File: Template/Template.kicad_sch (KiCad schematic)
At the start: 16 parts, among them J1 Conn_01x04, J2 Conn_01x04, J3 Conn_02x05_Odd_Even, J4 Conn_01x01, J6 Conn_02x05_Odd_Even, U1 PCA9535DBR

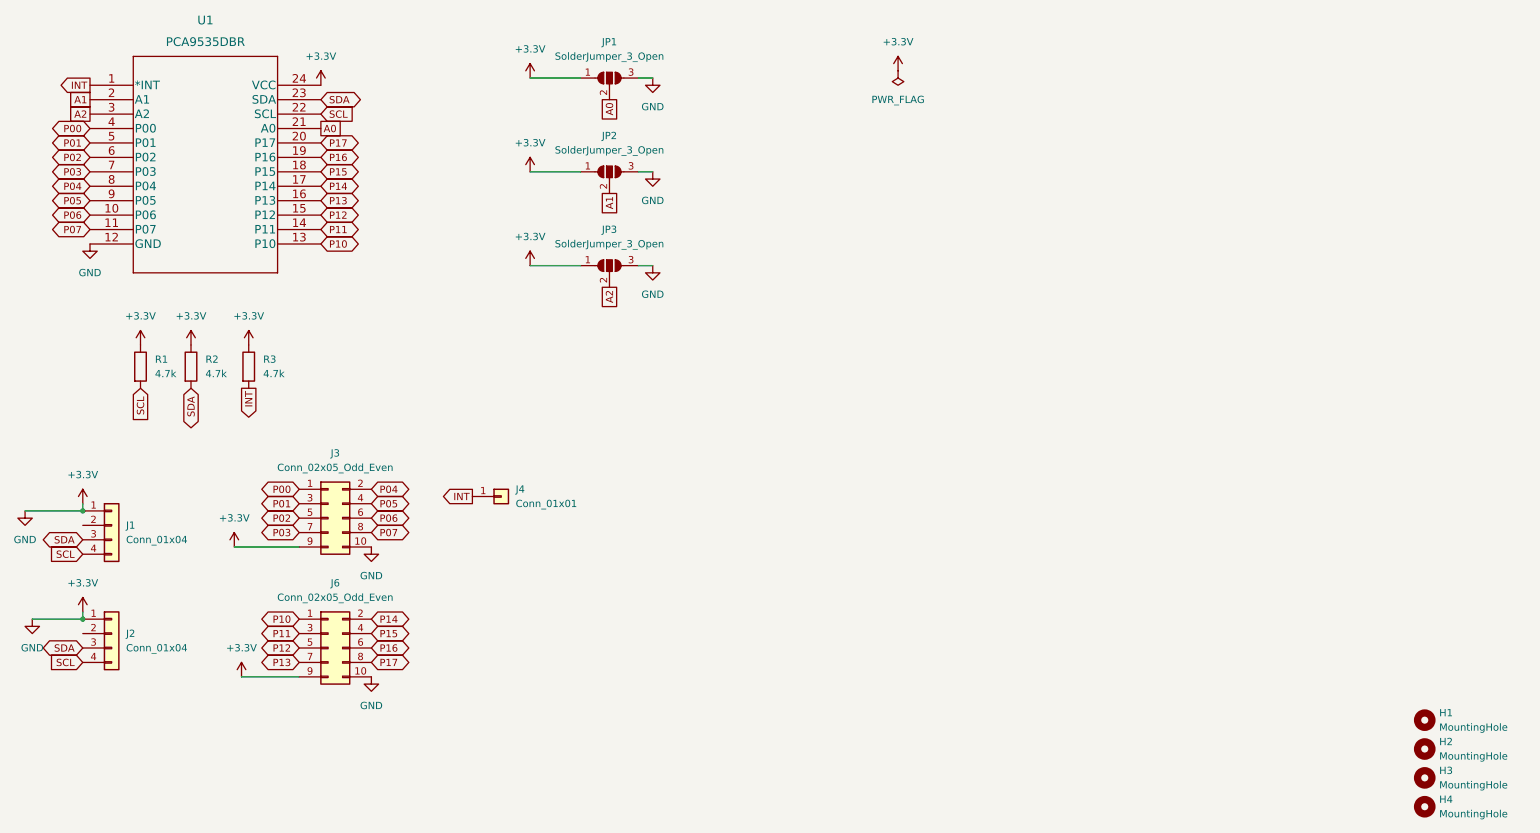
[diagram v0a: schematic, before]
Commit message: Futher Progress on the gpio
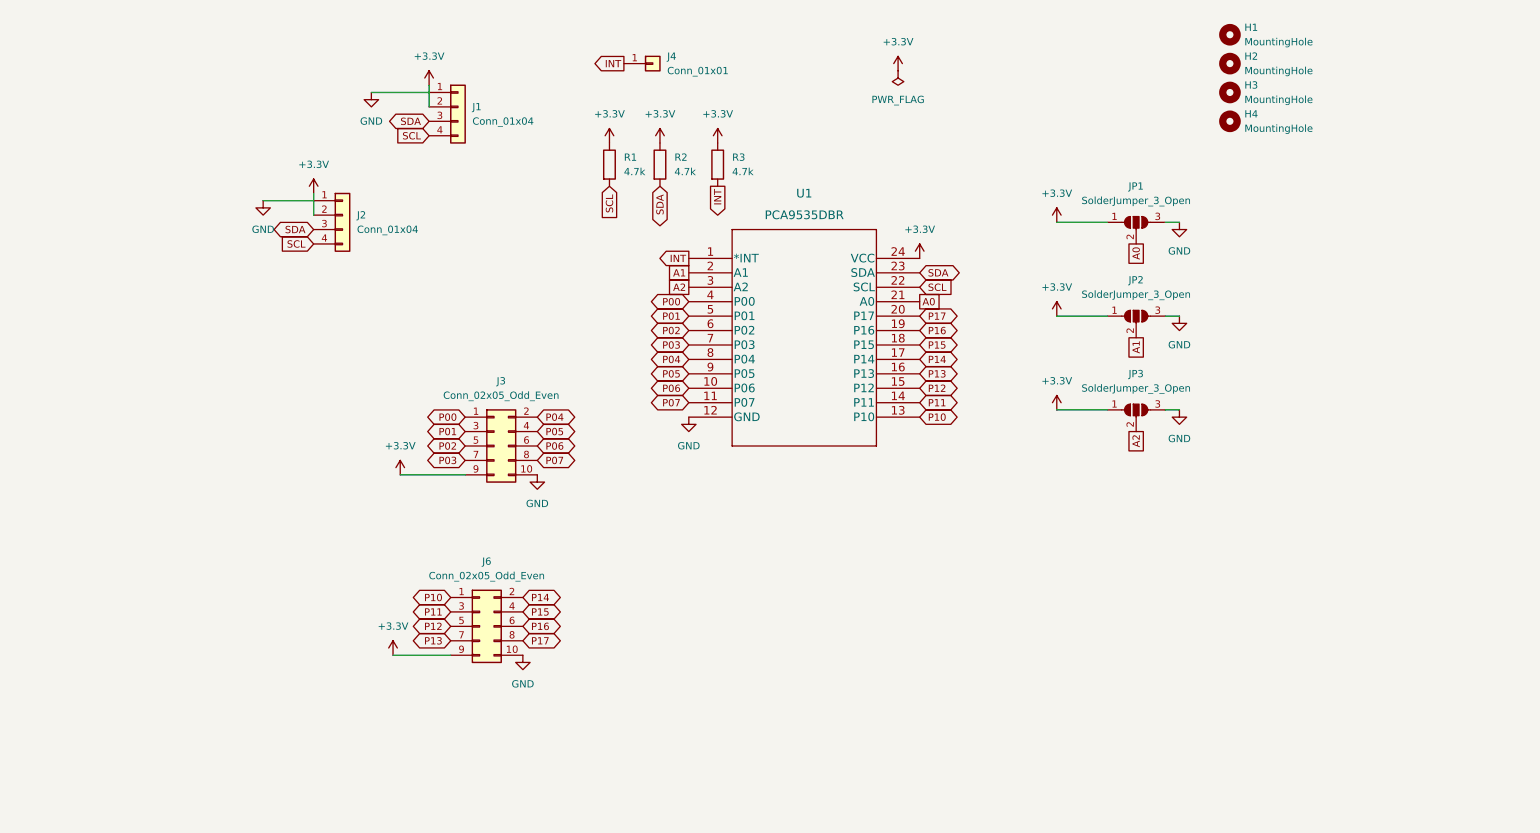
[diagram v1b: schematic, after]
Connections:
- net +3.3V: now also J1.2 (Pin_2), J2.2 (Pin_2); no longer J1.1 (Pin_1), J2.1 (Pin_1), J3.10 (Pin_10), J6.10 (Pin_10), JP1.3 (B), JP2.3 (B), JP3.3 (B), U1.12 (GND)
- new net GND: J1.1 (Pin_1), J2.1 (Pin_1), J3.10 (Pin_10), J6.10 (Pin_10), JP1.3 (B), JP2.3 (B), JP3.3 (B), U1.12 (GND)
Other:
- company: Because I'm Clever -> (none)
- title: 16pin GPIO Expander -> (none)
- moved on the sheet: H1, H2, H3, H4, J1, J2, J3, J4, J6, JP1, JP2, JP3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
